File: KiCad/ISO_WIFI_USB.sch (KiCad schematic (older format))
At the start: 27 parts, among them P6 CONN_02X03, P7 CONN_02X03, P8 USB_B, SW3 SWITCH_INV, T1 da2303, U19 TLV73333PDBVT, U35 ADUM1402BRWZ, U36 ISO7341c_spi, U40 CP2102N-24, U5 ESP-12F, U6 SN6505A

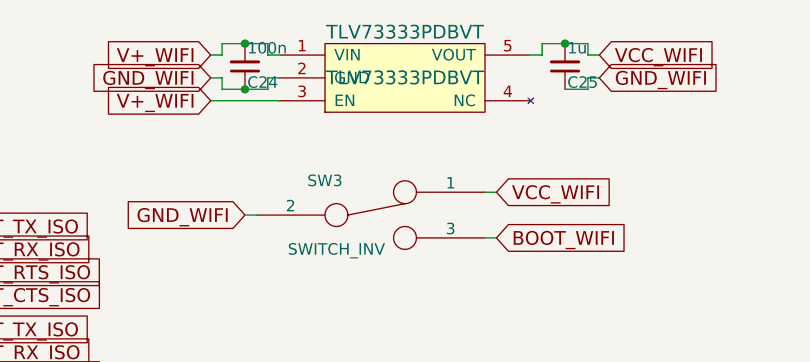
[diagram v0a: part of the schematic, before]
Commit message: kicad
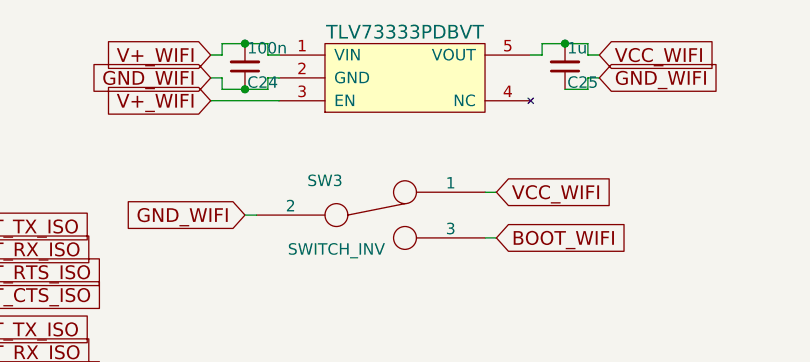
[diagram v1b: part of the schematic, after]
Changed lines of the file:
@@
 F 2 "TO_SOT_Packages_SMD:SOT-23-5" H 7000 1000 60  0001 C CNN
 F 3 "" H 7000 1000 60  0001 C CNN
-F 4 "TLV73333PDBVT" H 7000 1000 60  0000 C CNN "manf#"
+F 4 "TLV73333PDBVT" H 7000 1000 60  0001 C CNN "manf#"
 	1    7000 1000
 	1    0    0    -1
